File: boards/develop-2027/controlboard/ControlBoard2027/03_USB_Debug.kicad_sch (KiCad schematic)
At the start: 12 parts, among them J2 USB-C_DFU, J3 SWD_5pin, SW1 RESET, SW2 BOOT0_DFU, U5 USBLC6-2SC6

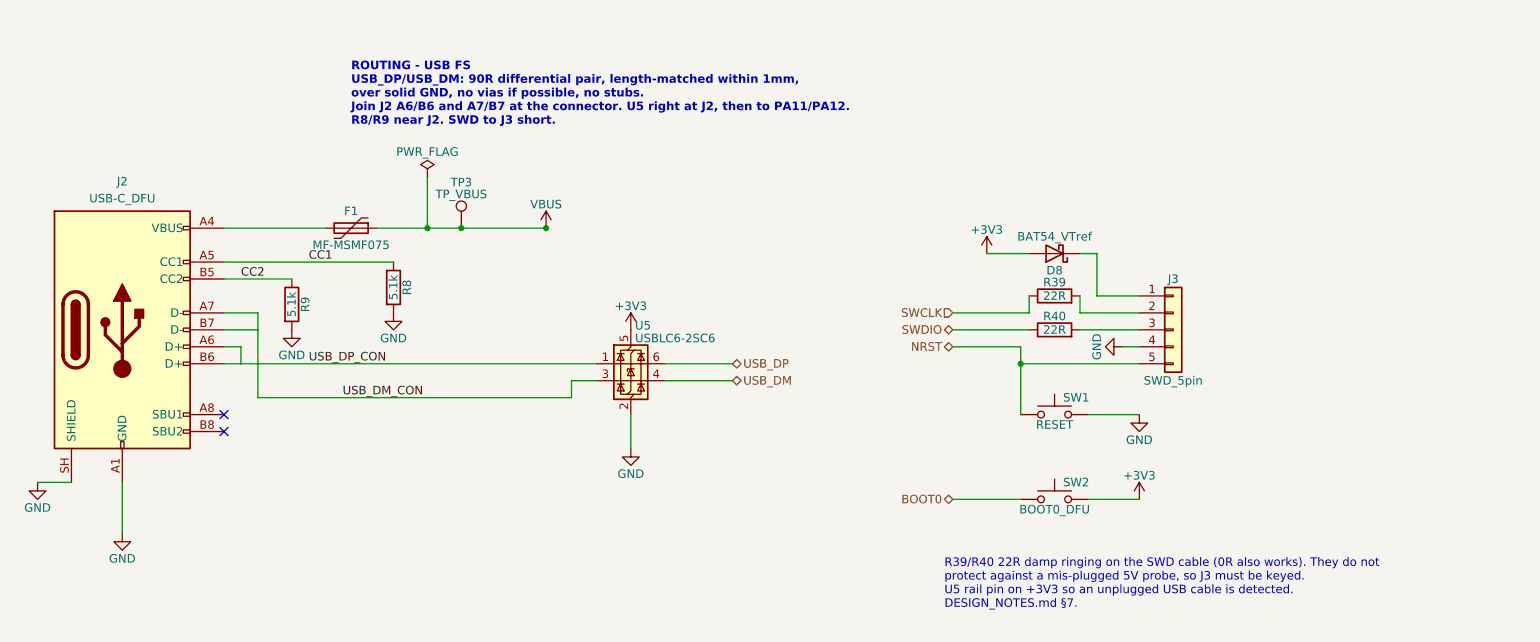
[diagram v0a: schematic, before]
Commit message: boxing goes brrr
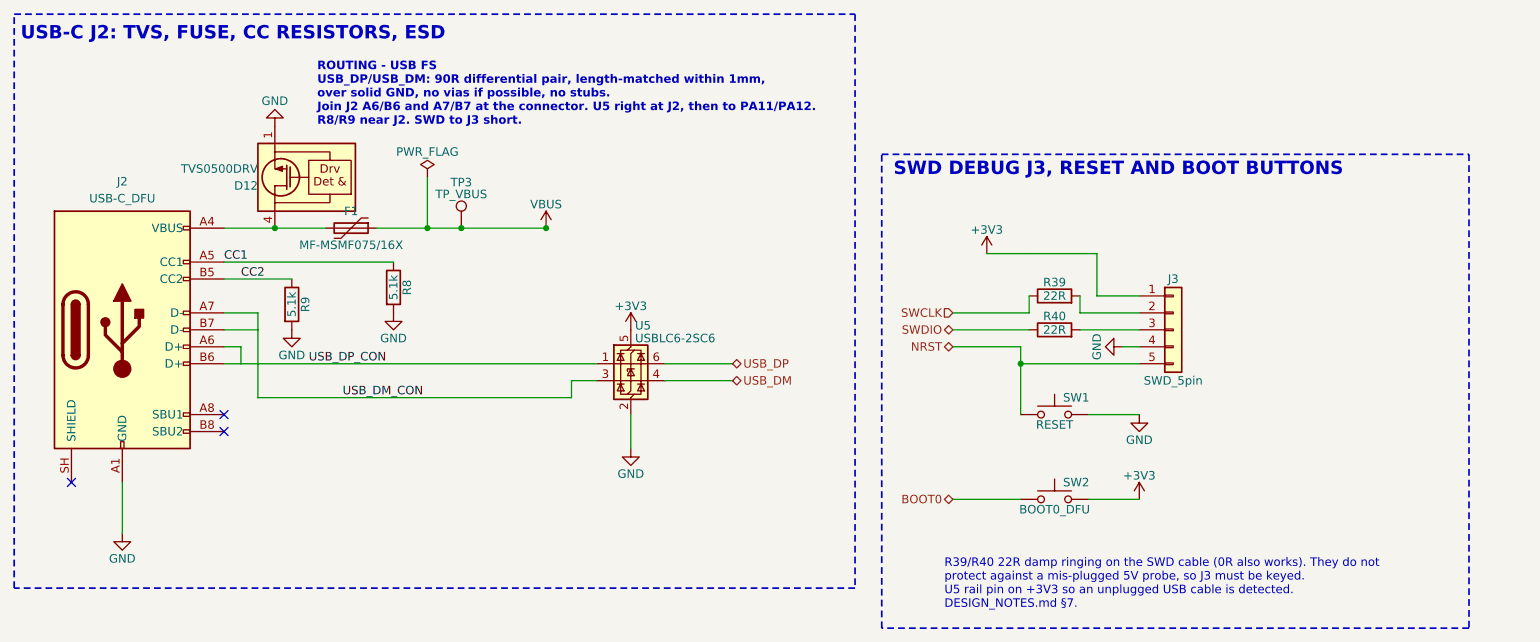
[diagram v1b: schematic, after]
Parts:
- removed D8: BAT54_VTref, symbol Device:D_Schottky
- added D12: TVS0500DRV, symbol Power_Protection:TVS0500DRV
- F1: value MF-MSMF075 -> MF-MSMF075/16X; MPN Bourns MF-MSMF075-2 -> Bourns MF-MSMF075/16X-2
- U5: MPN (none) -> ST USBLC6-2SC6
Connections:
- net +3V3: now also J3.1 (Pin_1)
- net GND: now also D12.1 (GND), D12.2 (GND), D12.3 (GND), D12.7 (GND); no longer J2.SH (SHIELD)
- net at F1.2, J2.A4 (VBUS), J2.A9 (VBUS)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: now also D12.4 (IN), D12.5 (IN), D12.6 (IN)
- no-connect marks 2 -> 3
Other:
- note added: "SWD DEBUG J3, RESET AND BOOT BUTTONS"
- note added: "USB-C J2: TVS, FUSE, CC RESISTORS, ESD"
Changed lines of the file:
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@@
 		(color 0 0 0 0)
+	)
+	(junction
+		(at 99.06 99.06)
+		(diameter 0)
 	)
 	(no_connect
@@
 		(at 91.44 129.54)
 	)
+	(no_connect
+		(at 68.58 137.16)
+	)
 	(wire
 		(pts
@@
 	(wire
 		(pts
-			(xy 68.58 137.16)
-			(xy 63.5 137.16)
-		)
-		(stroke
-			(width 0)
-			(type default)
-		)
-	)
-	(wire
-		(pts
 			(xy 219.71 114.3)
 			(xy 228.6 114.3)
@@
 		)
 	)
-	(text "ROUTING - USB FS\nUSB_DP/USB_DM: 90R differential pair, length-matched within 1mm,\nover solid GND, no vias if possible, no stubs.\nJoin J2 A6/B6 and A7/B7 at the connector. U5 right at J2, then to PA11/PA12.\nR8/R9 near J2. SWD to J3 short."
-		(at 110.49 83.82 0)
+	(wire
+		(pts
+			(xy 212.09 102.87)
+			(xy 219.71 102.87)
+		)
+	)
+	(text "R39/R40 22R damp ringing on the SWD cable (0R also works). They do not\nprotect against a mis-plugged 5V probe, so J3 must be keyed.\nU5 rail pin on +3V3 so an unplugged USB cable is detected.\nDESIGN_NOTES.md §7."
+		(at 199.39 156.21 0)
 		(effects
 			(font
 				(size 1.27 1.27)
-				(bold yes)
-				(color 255 0 0 1)
 			)
 			(justify left bottom)
@@
 	)
 	(label "CC1"
-		(at 104.14 104.14 0)
+		(at 91.44 104.14 0)
 		(effects
 			(font
@@
 		)
 	)
-  (text "R39/R40 22R damp ringing on the SWD cable (0R also works). They do not\nprotect against a mis-plugged 5V probe, so J3 must be keyed.\nU5 rail pin on +3V3 so an unplugged USB cable is detected.\nDESIGN_NOTES.md §7."
-    (at 199.39 156.21 0)
-    (effects (font (size 1.27 1.27)) (justify left bottom))
+  (text "ROUTING - USB FS\nUSB_DP/USB_DM: 90R differential pair, length-matched within 1mm,\nover solid GND, no vias if possible, no stubs.\nJoin J2 A6/B6 and A7/B7 at the connector. U5 right at J2, then to PA11/PA12.\nR8/R9 near J2. SWD to J3 short."
+    (at 105.41 83.82 0)
+    (effects (font (size 1.27 1.27) (bold yes) (color 255 0 0 1)) (justify left bottom))
+  )
+  (text "USB-C J2: TVS, FUSE, CC RESISTORS, ESD"
+    (at 60.96 71.12 0)
+    (effects (font (size 2 2) (thickness 0.4) (bold yes) (color 0 0 132 1)) (justify left bottom))
+  )
+  (text "SWD DEBUG J3, RESET AND BOOT BUTTONS"
+    (at 191.77 91.44 0)
+    (effects (font (size 2 2) (thickness 0.4) (bold yes) (color 0 0 132 1)) (justify left bottom))
   )
 	(symbol
@@
 			)
 		)
-		(property "Description" "GCT USB4110-GF-A, USB 2.0 Type-C 16P SMT receptacle. VBUS 5A total, GND 6.25A total, 0.25A per signal pin, 48VDC, 20,000 cycles. Same series as the rev-2026 control board (C5143397). Footprint pads match the symbol (A1-B12, SH)."
+		(property "Description" "GCT USB4110-GF-A, USB 2.0 Type-C 16P SMT receptacle. VBUS 5A total, GND 6.25A total, 0.25A per signal pin. Shield (SH) left floating by design choice."
 			(at 76.2 114.3 0)
 			(hide yes)
@@
 	)
 	(symbol
-		(lib_id "Device:D_Schottky")
-		(at 215.9 102.87 180)
-		(unit 1)
-		(exclude_from_sim no)
-		(in_bom yes)
-		(on_board yes)
-		(dnp no)
-		(property "Reference" "D8"
-			(at 215.9 105.41 0)
-			(show_name no)
-			(do_not_autoplace no)
-			(effects
-				(font
-					(size 1.27 1.27)
-				)
-			)
-		)
-		(property "Value" "BAT54_VTref"
-			(at 215.9 100.33 0)
-			(show_name no)
-			(do_not_autoplace no)
-			(effects
-				(font
-					(size 1.27 1.27)
-				)
-			)
-		)
-		(property "Footprint" ""
-			(at 215.9 102.87 0)
-			(hide yes)
-			(show_name no)
-			(do_not_autoplace no)
-			(effects
-				(font
-					(size 1.27 1.27)
-				)
-			)
-		)
-		(property "Datasheet" ""
-			(at 215.9 102.87 0)
-			(hide yes)
-			(show_name no)
-			(do_not_autoplace no)
-			(effects
-				(font
-					(size 1.27 1.27)
-				)
-			)
-		)
-		(property "Description" "Schottky diode"
-			(at 215.9 102.87 0)
-			(hide yes)
-			(show_name no)
-			(do_not_autoplace no)
-			(effects
-				(font
-					(size 1.27 1.27)
-				)
-			)
-		)
-		(body_style 1)
-		(in_pos_files yes)
-		(pin "1"
-		)
-		(pin "2"
-		)
-		(instances
-			(project "ControlBoard2027"
-				(path "/2be89789-dd04-494d-960d-2531c7ce8a2f/b44198b9-a21d-475d-9b21-d8da342bbbd1"
-					(reference "D8")
-					(unit 1)
-				)
-			)
-		)
-	)
-	(symbol
 		(lib_id "Device:R")
 		(at 116.84 107.95 0)
@@
 			)
 		)
-	)
+		(property "MPN" "ST USBLC6-2SC6"
+			(at 152.4 119.38 0)
+			(hide yes)
+			(effects
+				(font
+					(size 1.27 1.27)
+				)
+			)
+		))
 	(symbol
 		(lib_id "Device:R")
@@
 	)
 	(symbol
-		(lib_id "power:GND")
-		(at 63.5 137.16 0)
-		(unit 1)
-		(exclude_from_sim no)
-		(in_bom yes)
-		(on_board yes)
-		(dnp no)
-		(property "Reference" "#PWR301"
-			(at 63.5 143.51 0)
-			(hide yes)
-			(show_name no)
-			(do_not_autoplace no)
-			(effects
-				(font
-					(size 1.27 1.27)
-				)
-			)
-		)
-		(property "Value" "GND"
-			(at 63.5 140.97 0)
-			(show_name no)
-			(do_not_autoplace no)
-			(effects
-				(font
-					(size 1.27 1.27)
-				)
-			)
-		)
-		(property "Footprint" ""
-			(at 63.5 137.16 0)
-			(hide yes)
-			(show_name no)
-			(do_not_autoplace no)
-			(effects
-				(font
-					(size 1.27 1.27)
-				)
-			)
-		)
-		(property "Datasheet" ""
-			(at 63.5 137.16 0)
-			(hide yes)
-			(show_name no)
-			(do_not_autoplace no)
-			(effects
-				(font
-					(size 1.27 1.27)
-				)
-			)
-		)
-		(property "Description" "Power symbol creates a global label with name \"GND\" , ground"
-			(at 63.5 137.16 0)
-			(hide yes)
-			(show_name no)
-			(do_not_autoplace no)
-			(effects
-				(font
-					(size 1.27 1.27)
-				)
-			)
-		)
-		(body_style 1)
-		(in_pos_files yes)
-		(pin "1"
-		)
-		(instances
-			(project "ControlBoard2027"
-				(path "/2be89789-dd04-494d-960d-2531c7ce8a2f/b44198b9-a21d-475d-9b21-d8da342bbbd1"
-					(reference "#PWR301")
-					(unit 1)
-				)
-			)
-		)
-	)
-	(symbol
 		(lib_id "Device:Polyfuse")
 		(at 110.49 99.06 270)
@@
 			)
 		)
-		(property "Value" "MF-MSMF075"
+		(property "Value" "MF-MSMF075/16X"
 			(at 110.49 101.6 90)
 			(show_name no)
@@
 			)
 		)
-		(property "Description" "Bourns MF-MSMF075-2 PTC, 1812, on USB VBUS. Ihold 0.75A / Itrip 1.50A at 23C, 0.60A hold at 50C, R 0.11-0.45 Ohm (Bourns derating table). U13 limits USB current to 0.455-0.560A first; F1 is backup for a U13 or cable short. MF-MSMF050 was replaced because its 0.40A hold at 50C tripped below U13's limit."
+		(property "Description" "USB VBUS PTC, 1812. Ihold 0.75A / Itrip 1.50A at 23C, 0.55A hold at 50C, 0.11-0.45 Ohm, 8A trips in 0.2s max (Bourns MF-MSMF Rev BD). Holds a USB 2.0 port's 0.5A and trips on a board or cable short. Motor modules on USB may trip it (DESIGN_NOTES.md §7)."
 			(at 110.49 99.06 0)
 			(hide yes)
@@
 			)
 		)
-		(property "MPN" "Bourns MF-MSMF075-2"
+		(property "MPN" "Bourns MF-MSMF075/16X-2"
 			(at 110.49 99.06 0)
 			(hide yes)
@@
 		)
 	)
+	(symbol
+		(lib_id "Power_Protection:TVS0500DRV")
+		(at 99.06 91.44 180)
+		(unit 1)
+		(in_bom yes)
+		(on_board yes)
+		(dnp no)
+		(property "Reference" "D12"
+			(at 96.52 92.71 0)
+			(effects
+				(font
+					(size 1.27 1.27)
+				)
+				(justify left)
+			)
+		)
+		(property "Value" "TVS0500DRV"
+			(at 96.52 90.17 0)
+			(effects
+				(font
+					(size 1.27 1.27)
+				)
+				(justify left)
+			)
+		)
+		(property "Footprint" ""
+			(at 99.06 91.44 0)
+			(hide yes)
+			(effects
+				(font
+					(size 1.27 1.27)
+				)
+			)
+		)
+		(property "Datasheet" "http://www.ti.com/lit/ds/symlink/tvs0500.pdf"
+			(at 99.06 91.44 0)
+			(hide yes)
+			(effects
+				(font
+					(size 1.27 1.27)
+				)
+			)
+		)
+		(property "Description" "USB VBUS TVS at J2, same part as D9/D10. TVS0500: VRWM 5V, VBR 7.5-8.4V, flat clamp 9.2V at 43A. Place right at J2 VBUS pins with a short GND via."
+			(at 99.06 91.44 0)
+			(hide yes)
+			(effects
+				(font
+					(size 1.27 1.27)
+				)
+			)
+		)
+		(instances
+			(project "ControlBoard2027"
+				(path "/2be89789-dd04-494d-960d-2531c7ce8a2f/b44198b9-a21d-475d-9b21-d8da342bbbd1"
+					(reference "D12")
+					(unit 1)
+				)
+			)
+		)
+		(property "MPN" "TI TVS0500DRVR"
+			(at 99.06 91.44 0)
+			(hide yes)
+			(effects
+				(font
+					(size 1.27 1.27)
+				)
+			)
+		))
+	(symbol
+		(lib_id "power:GND")
+		(at 99.06 83.82 180)
+		(unit 1)
+		(in_bom yes)
+		(on_board yes)
+		(dnp no)
+		(property "Reference" "#PWR313"
+			(at 99.06 77.47 0)
+			(hide yes)
+			(effects
+				(font
+					(size 1.27 1.27)
+				)
+			)
+		)
+		(property "Value" "GND"
+			(at 99.06 80.01 0)
+			(effects
+				(font
+					(size 1.27 1.27)
+				)
+			)
+		)
+		(property "Footprint" ""
+			(at 99.06 83.82 0)
+			(hide yes)
+			(effects
+				(font
+					(size 1.27 1.27)
+				)
+			)
+		)
+		(property "Datasheet" ""
+			(at 99.06 83.82 0)
+			(hide yes)
+			(effects
+				(font
+					(size 1.27 1.27)
+				)
+			)
+		)
+		(property "Description" "Power symbol creates a global label with name \"GND\" , ground"
+			(at 99.06 83.82 0)
+			(hide yes)
+			(effects
+				(font
+					(size 1.27 1.27)
+				)
+			)
+		)
+		(instances
+			(project "ControlBoard2027"
+				(path "/2be89789-dd04-494d-960d-2531c7ce8a2f/b44198b9-a21d-475d-9b21-d8da342bbbd1"
+					(reference "#PWR313")
+					(unit 1)
+				)
+			)
+		)
+	)
+	(rectangle
+		(start 60 67)
+		(end 186 153)
+		(stroke
+			(width 0.254)
+			(type dash)
+			(color 0 0 132 1)
+		)
+		(fill
+			(type none)
+		)
+	)
+	(rectangle
+		(start 190 88)
+		(end 278 159)
+		(stroke
+			(width 0.254)
+			(type dash)
+			(color 0 0 132 1)
+		)
+		(fill
+			(type none)
+		)
+	)
